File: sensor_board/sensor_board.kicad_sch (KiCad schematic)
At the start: 4 parts, among them U1 TSL25911FN

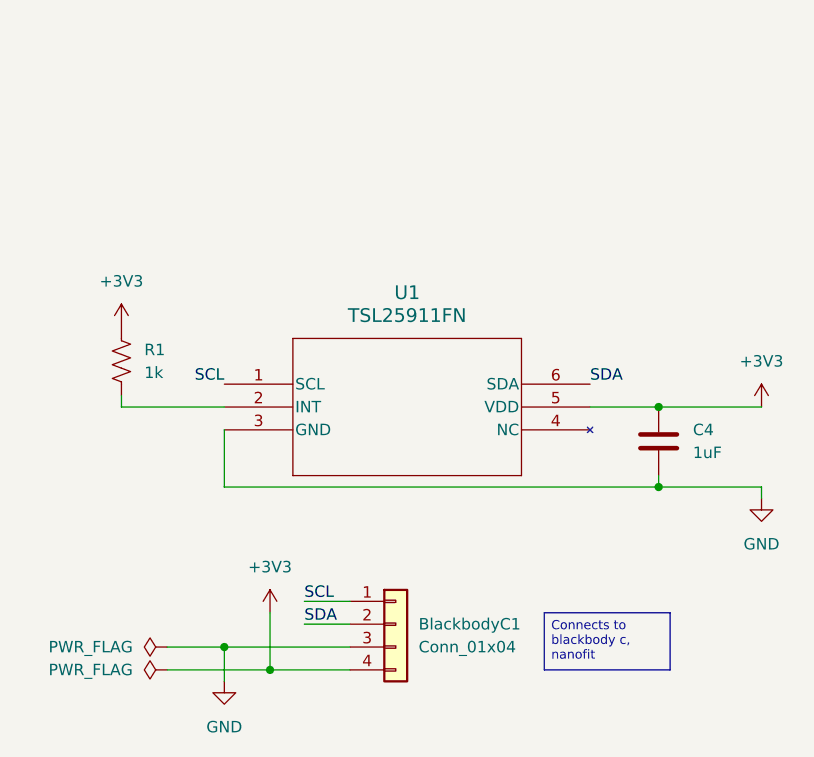
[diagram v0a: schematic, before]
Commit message: layout updates
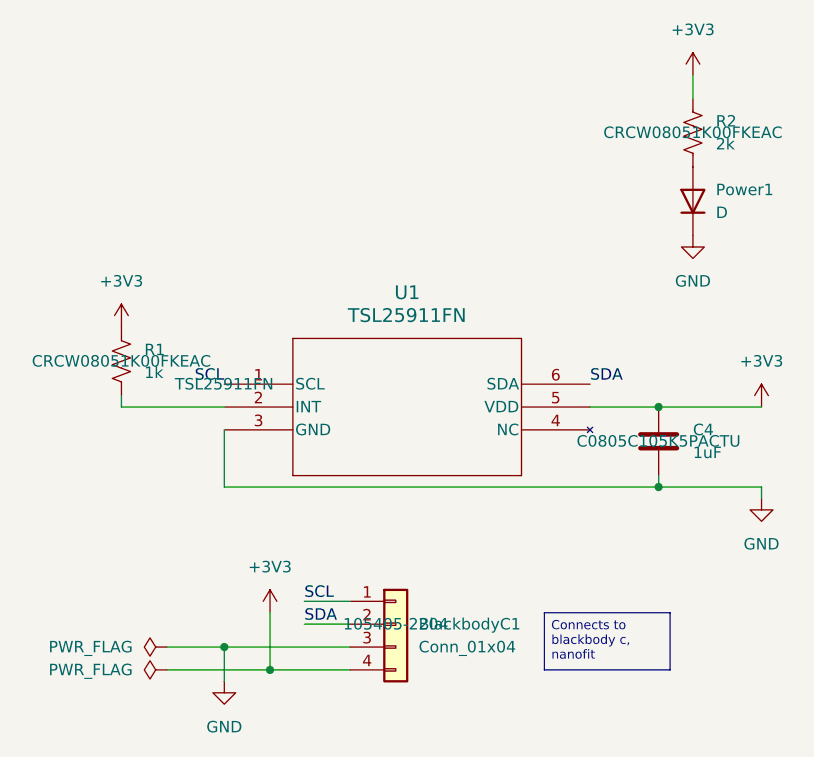
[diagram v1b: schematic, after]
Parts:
- added Power1: D, LED_SMD:LED_0805_2012Metric, symbol Device:D
- added R2: 2k, Resistor_SMD:R_0805_2012Metric, symbol Device:R_US
- BlackbodyC1: PN (none) -> 105405-2204
- C4: footprint Capacitor_SMD:C_0402_1005Metric -> Capacitor_SMD:C_0805_2012Metric; PN (none) -> C0805C105K5PACTU
- R1: footprint Resistor_SMD:R_0402_1005Metric -> Resistor_SMD:R_0805_2012Metric; PN (none) -> CRCW08051K00FKEAC
- U1: PN (none) -> TSL25911FN
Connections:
- net +3V3: now also R2.1
- net GND: now also Power1.1 (K)
- new net: Power1.2 (A), R2.2
